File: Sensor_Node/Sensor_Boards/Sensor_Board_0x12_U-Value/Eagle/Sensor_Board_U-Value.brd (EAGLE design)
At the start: 31.5 x 57 mm, 25 parts, among them IC1 MCP3911A0-E/SS, IC2 4066D, J2 ARDUINO_ISP, U2 ATMEGA328P_TQFP, Y1 8MHZ

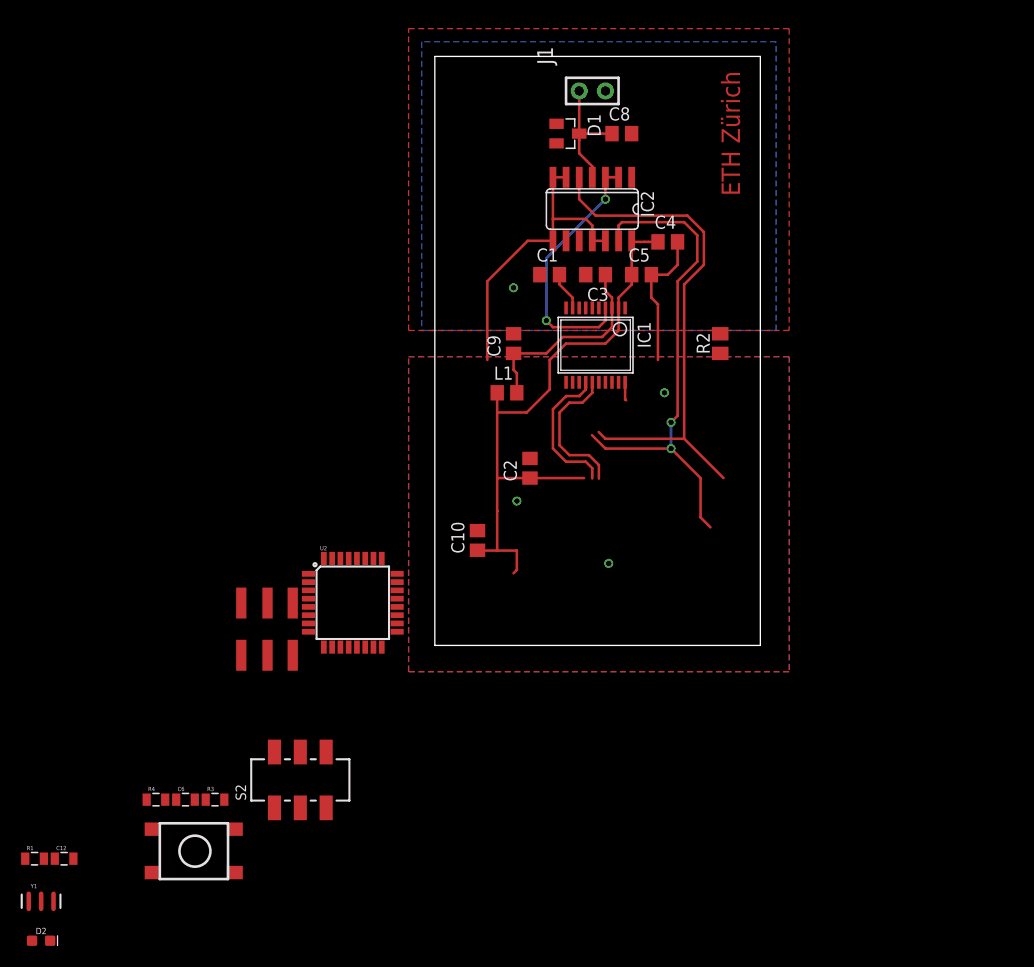
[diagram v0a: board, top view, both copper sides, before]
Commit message: Added WSN eagle library
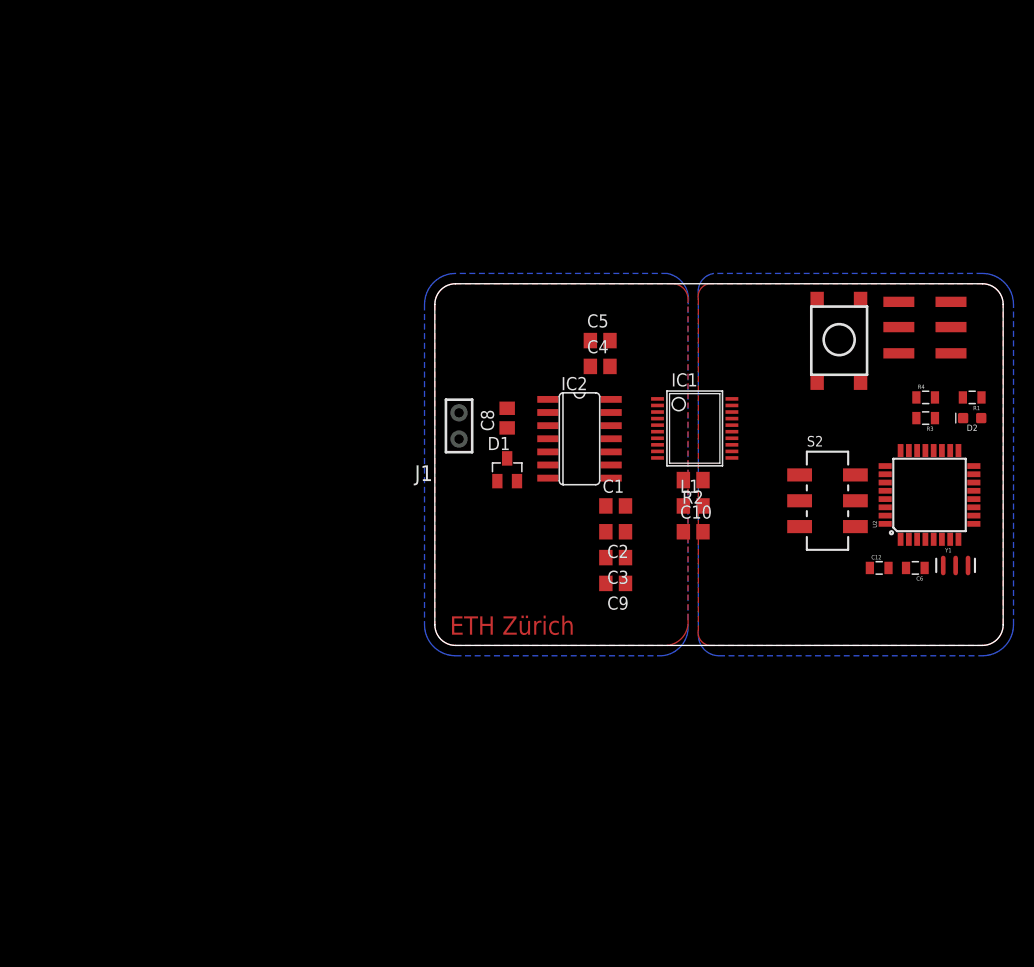
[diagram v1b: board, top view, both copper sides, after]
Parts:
- moved D2 103.3 mm to (52.0, 22.0), turned to 180 degrees
- moved R1 101.1 mm to (52.0, 24.0), turned to 180 degrees
- moved Y1 94.3 mm to (50.4, 7.74)
- moved R4 84.0 mm to (47.5, 24.0)
- moved C12 83.7 mm to (43.0, 7.50)
- moved R3 78.1 mm to (47.5, 22.0), turned to 180 degrees
- moved S3 77.5 mm to (37.0, 25.5), turned to 90 degrees
- moved J2 74.6 mm to (50.0, 28.3), turned to 90 degrees
- moved C6 74.1 mm to (46.5, 7.50), turned to 180 degrees
- moved S2 57.7 mm to (38.0, 14.0), turned to 270 degrees
- moved U2 56.8 mm to (47.9, 14.6), turned to 90 degrees
- moved J1 34.2 mm to (2.34, 22.5), turned to 180 degrees
- moved D1 33.1 mm to (7.00, 17.0), turned to 0 degrees
- moved C8 29.7 mm to (7.00, 22.0), turned to 90 degrees
- moved C3 27.4 mm to (17.5, 8.50)
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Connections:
- removed net D11_MOSI: U2.15
- removed net D12_MISO: J2.P$1, J2.P$3, U2.16
- removed net D13_SCK: J2.P$2, U2.17
- removed net N$16: U2.32
- removed net N$20: U2.10
- removed net N$21: U2.11
- net ADCLK: now also U2.32
- net AD_CS: now also U2.10
- net DATA_READY: now also U2.11
- net MISO: now also J2.P$1, U2.16
- net MOSI: now also J2.P$3, U2.15
- net SCK: now also J2.P$2, U2.17
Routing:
- net DVDD: track 58.3 -> 0.00 mm
- net INPUT_EN: track 50.2 -> 0.00 mm
- net SHORT: track 48.8 -> 0.00 mm, vias 2 -> 0
- net DGND: track 43.5 -> 0.00 mm, vias 3 -> 0
- net N$8: track 25.0 -> 0.00 mm, vias 2 -> 0
- net AVDD: track 19.9 -> 0.00 mm
- net ADCLK: track 14.1 -> 0.00 mm
- net DATA_READY: track 14.1 -> 0.00 mm
- net N$12: track 12.1 -> 0.00 mm
- net N$2: track 3.74 -> 0.00 mm
- net MOSI: track 2.08 -> 0.00 mm
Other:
- board size 31.5 x 57 mm -> 55 x 35 mm
